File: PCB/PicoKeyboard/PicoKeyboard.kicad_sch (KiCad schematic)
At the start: 1 part, among them U1 Raspberry_Pi_Pico

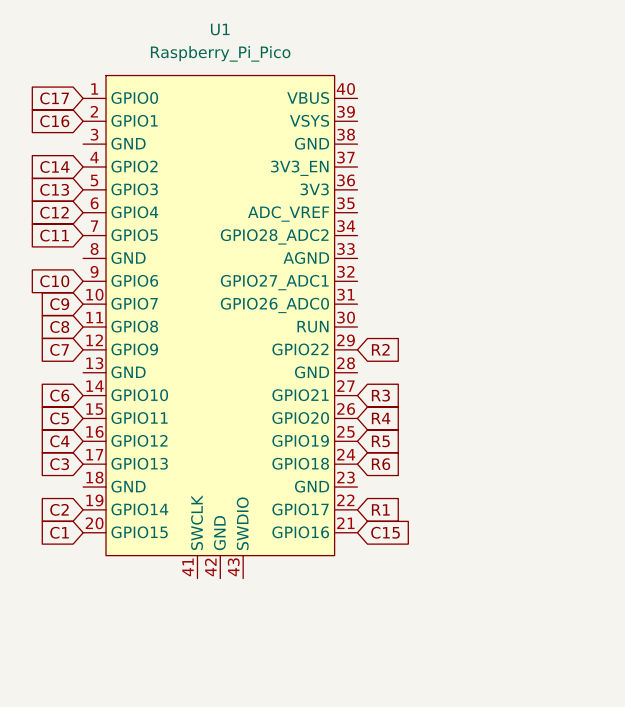
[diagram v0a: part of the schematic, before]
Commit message: Rewired
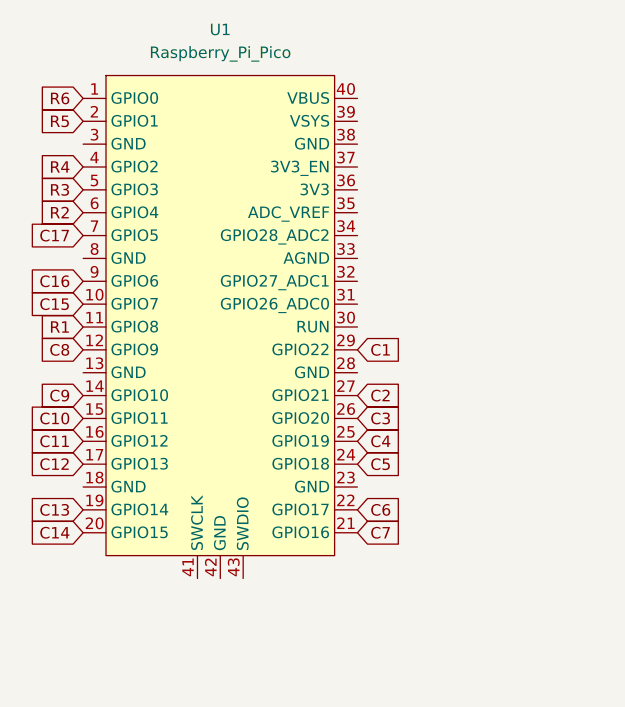
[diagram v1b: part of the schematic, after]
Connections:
- net C1: now also U1.29 (GPIO22); no longer U1.20 (GPIO15)
- net C10: now also U1.15 (GPIO11); no longer U1.9 (GPIO6)
- net C11: now also U1.16 (GPIO12); no longer U1.7 (GPIO5)
- net C12: now also U1.17 (GPIO13); no longer U1.6 (GPIO4)
- net C13: now also U1.19 (GPIO14); no longer U1.5 (GPIO3)
- net C14: now also U1.20 (GPIO15); no longer U1.4 (GPIO2)
- net C15: now also U1.10 (GPIO7); no longer U1.21 (GPIO16)
- net C16: now also U1.9 (GPIO6); no longer U1.2 (GPIO1)
- net C17: now also U1.7 (GPIO5); no longer U1.1 (GPIO0)
- net C2: now also U1.27 (GPIO21); no longer U1.19 (GPIO14)
- net C3: now also U1.26 (GPIO20); no longer U1.17 (GPIO13)
- net C4: now also U1.25 (GPIO19); no longer U1.16 (GPIO12)
- net C5: now also U1.24 (GPIO18); no longer U1.15 (GPIO11)
- net C6: now also U1.22 (GPIO17); no longer U1.14 (GPIO10)
- net C7: now also U1.21 (GPIO16); no longer U1.12 (GPIO9)
- net C8: now also U1.12 (GPIO9); no longer U1.11 (GPIO8)
- net C9: now also U1.14 (GPIO10); no longer U1.10 (GPIO7)
- net R1: now also U1.11 (GPIO8); no longer U1.22 (GPIO17)
- net R2: now also U1.6 (GPIO4); no longer U1.29 (GPIO22)
- net R3: now also U1.5 (GPIO3); no longer U1.27 (GPIO21)
- net R4: now also U1.4 (GPIO2); no longer U1.26 (GPIO20)
- net R5: now also U1.2 (GPIO1); no longer U1.25 (GPIO19)
- net R6: now also U1.1 (GPIO0); no longer U1.24 (GPIO18)

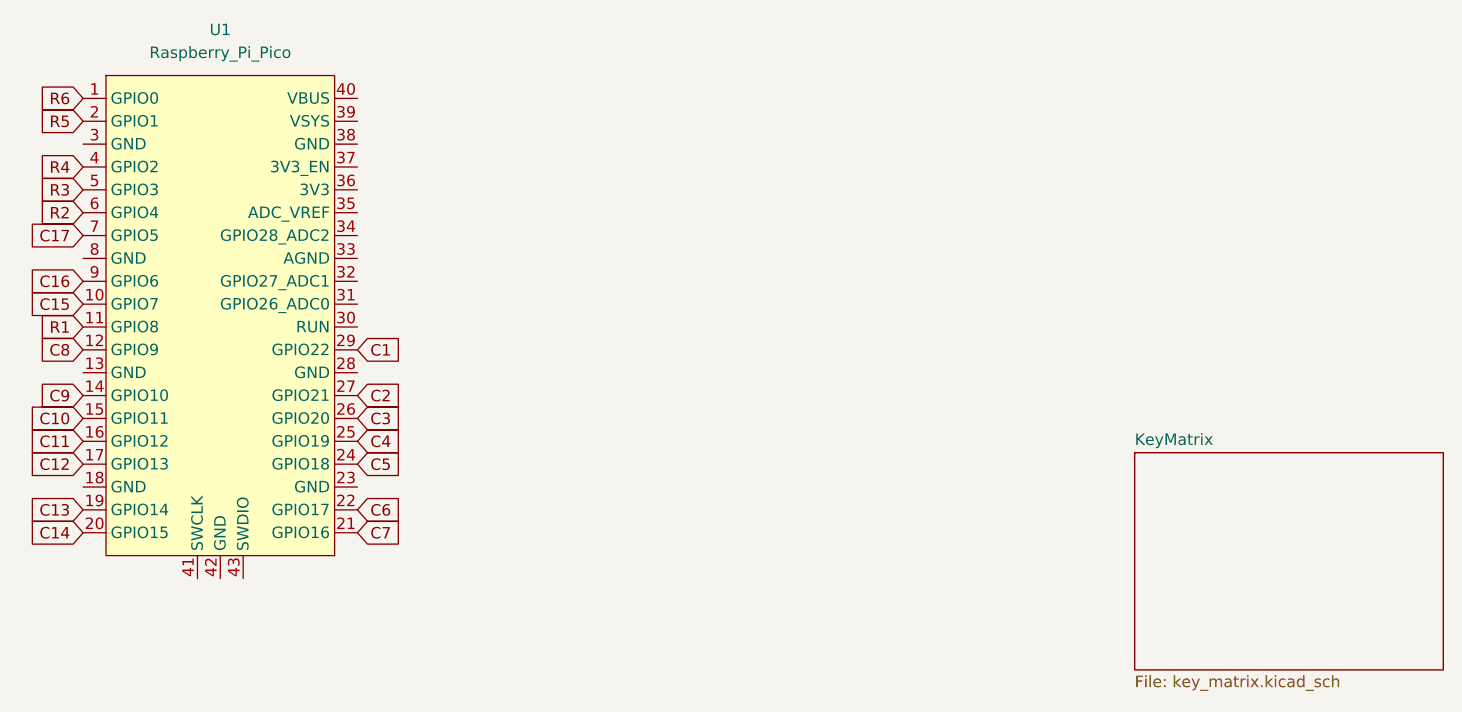
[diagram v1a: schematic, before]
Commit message: New layout
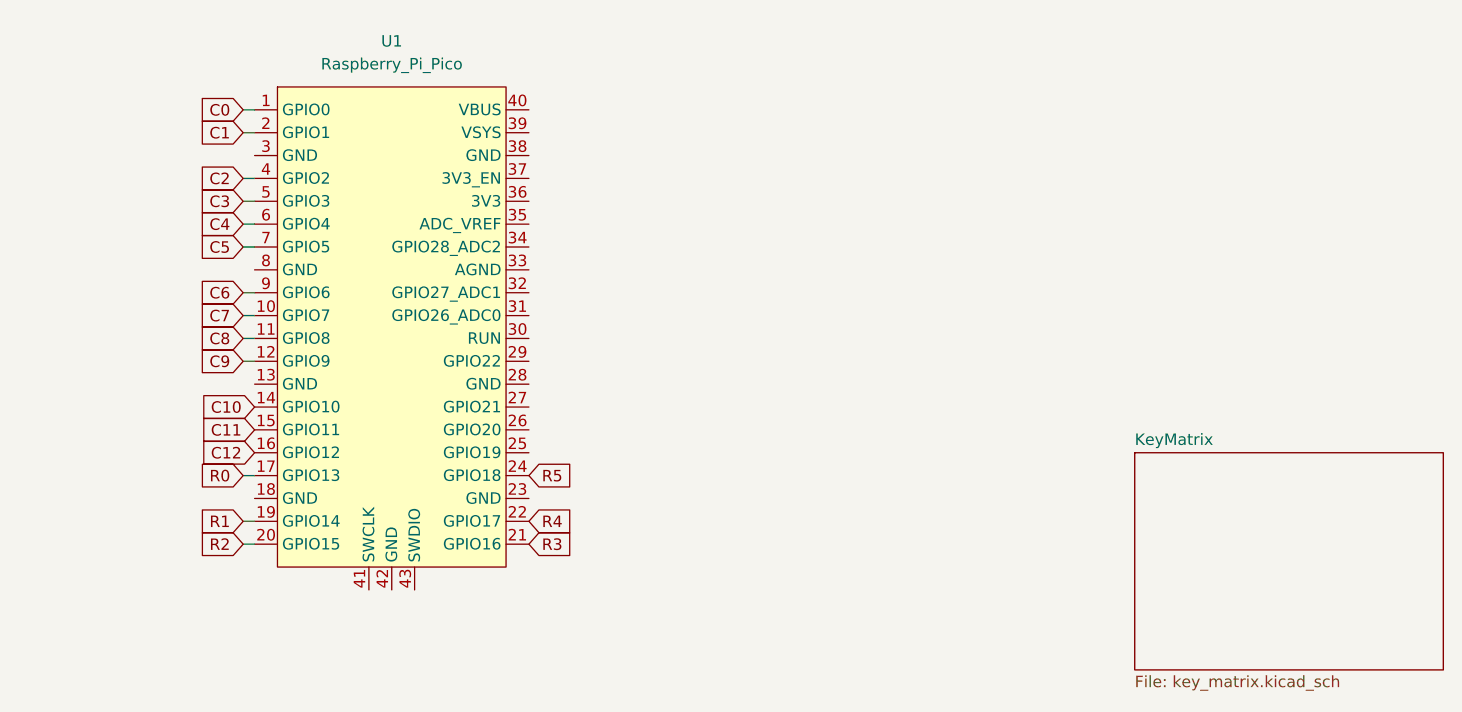
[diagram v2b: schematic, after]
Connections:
- net C13 is gone; now on net R1: U1.19 (GPIO14)
- net C14 is gone; now on net R2: U1.20 (GPIO15)
- net C15 is gone; now on net C7: U1.10 (GPIO7)
- net C16 is gone; now on net C6: U1.9 (GPIO6)
- net C17 is gone; now on net C5: U1.7 (GPIO5)
- net C1: now also U1.2 (GPIO1); no longer U1.29 (GPIO22)
- net C10: now also U1.14 (GPIO10); no longer U1.15 (GPIO11)
- net C11: now also U1.15 (GPIO11); no longer U1.16 (GPIO12)
- net C12: now also U1.16 (GPIO12); no longer U1.17 (GPIO13)
- net C2: now also U1.4 (GPIO2); no longer U1.27 (GPIO21)
- net C3: now also U1.5 (GPIO3); no longer U1.26 (GPIO20)
- net C4: now also U1.6 (GPIO4); no longer U1.25 (GPIO19)
- net C5: no longer U1.24 (GPIO18)
- net C6: no longer U1.22 (GPIO17)
- net C7: no longer U1.21 (GPIO16)
- net C8: now also U1.11 (GPIO8); no longer U1.12 (GPIO9)
- net C9: now also U1.12 (GPIO9); no longer U1.14 (GPIO10)
- net R1: no longer U1.11 (GPIO8)
- net R2: no longer U1.6 (GPIO4)
- net R3: now also U1.21 (GPIO16); no longer U1.5 (GPIO3)
- net R4: now also U1.22 (GPIO17); no longer U1.4 (GPIO2)
- net R5: now also U1.24 (GPIO18); no longer U1.2 (GPIO1)
- net R6 renamed C0
- new net R0: U1.17 (GPIO13)
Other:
- moved on the sheet: U1

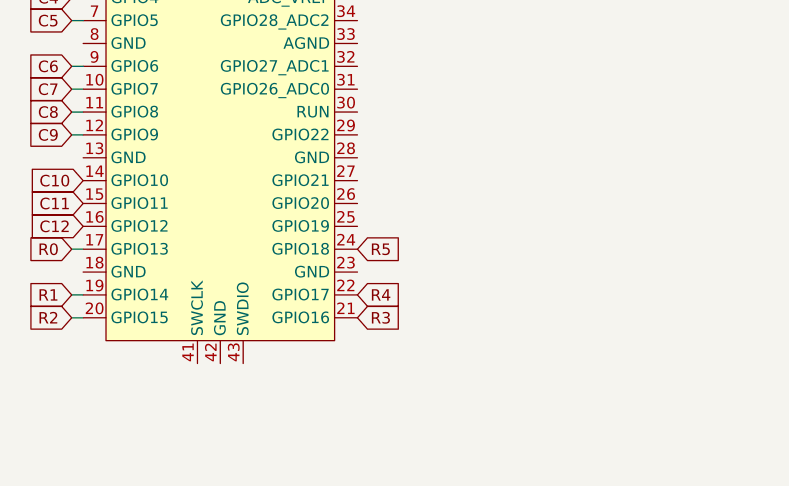
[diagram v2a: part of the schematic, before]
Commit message: Complete wiring
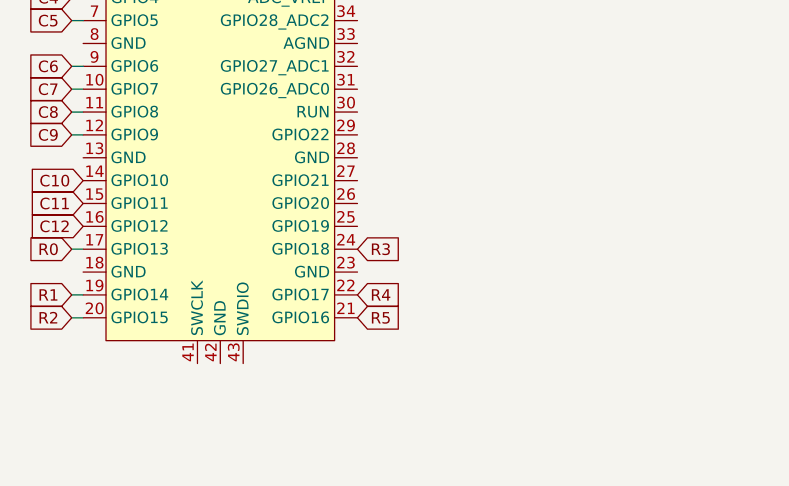
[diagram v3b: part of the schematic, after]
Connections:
- net R3: now also U1.24 (GPIO18); no longer U1.21 (GPIO16)
- net R5: now also U1.21 (GPIO16); no longer U1.24 (GPIO18)
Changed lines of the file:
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@@
 	(global_label "R5"
 		(shape input)
-		(at 137.16 100.33 0)
+		(at 137.16 107.95 0)
 		(fields_autoplaced yes)
 		(effects
@@
 		)
 		(property "Intersheetrefs" "${INTERSHEET_REFS}"
-			(at 142.6247 100.33 0)
+			(at 142.6247 107.95 0)
 			(effects
 				(font
@@
 	(global_label "R3"
 		(shape input)
-		(at 137.16 107.95 0)
+		(at 137.16 100.33 0)
 		(fields_autoplaced yes)
 		(effects
@@
 		)
 		(property "Intersheetrefs" "${INTERSHEET_REFS}"
-			(at 142.6247 107.95 0)
+			(at 142.6247 100.33 0)
 			(effects
 				(font

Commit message: Change layout
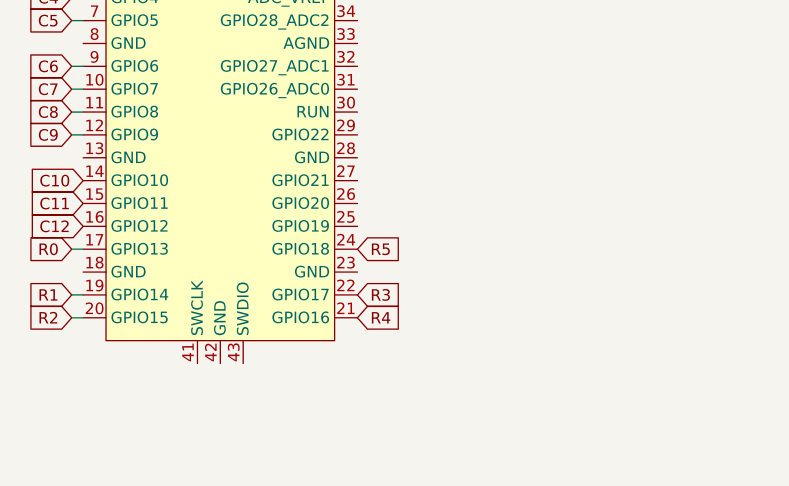
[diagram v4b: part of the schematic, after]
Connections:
- net R3: now also U1.22 (GPIO17); no longer U1.24 (GPIO18)
- net R4: now also U1.21 (GPIO16); no longer U1.22 (GPIO17)
- net R5: now also U1.24 (GPIO18); no longer U1.21 (GPIO16)
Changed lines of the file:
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@@
 	(global_label "R4"
 		(shape input)
-		(at 137.16 105.41 0)
+		(at 137.16 107.95 0)
 		(fields_autoplaced yes)
 		(effects
@@
 		)
 		(property "Intersheetrefs" "${INTERSHEET_REFS}"
-			(at 142.6247 105.41 0)
+			(at 142.6247 107.95 0)
 			(effects
 				(font
@@
 	(global_label "R5"
 		(shape input)
-		(at 137.16 107.95 0)
+		(at 137.16 100.33 0)
 		(fields_autoplaced yes)
 		(effects
@@
 		)
 		(property "Intersheetrefs" "${INTERSHEET_REFS}"
-			(at 142.6247 107.95 0)
+			(at 142.6247 100.33 0)
 			(effects
 				(font
@@
 	(global_label "R3"
 		(shape input)
-		(at 137.16 100.33 0)
+		(at 137.16 105.41 0)
 		(fields_autoplaced yes)
 		(effects
@@
 		)
 		(property "Intersheetrefs" "${INTERSHEET_REFS}"
-			(at 142.6247 100.33 0)
+			(at 142.6247 105.41 0)
 			(effects
 				(font
